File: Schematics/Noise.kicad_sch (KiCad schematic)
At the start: 46 parts, among them J72 Conn_01x04, J73 Conn_01x04, J74 Conn_01x04, Q10 BC547, Q7 BC547, Q8 BC547, Q9 BC547, U116 ADG419BN, U117 TL074

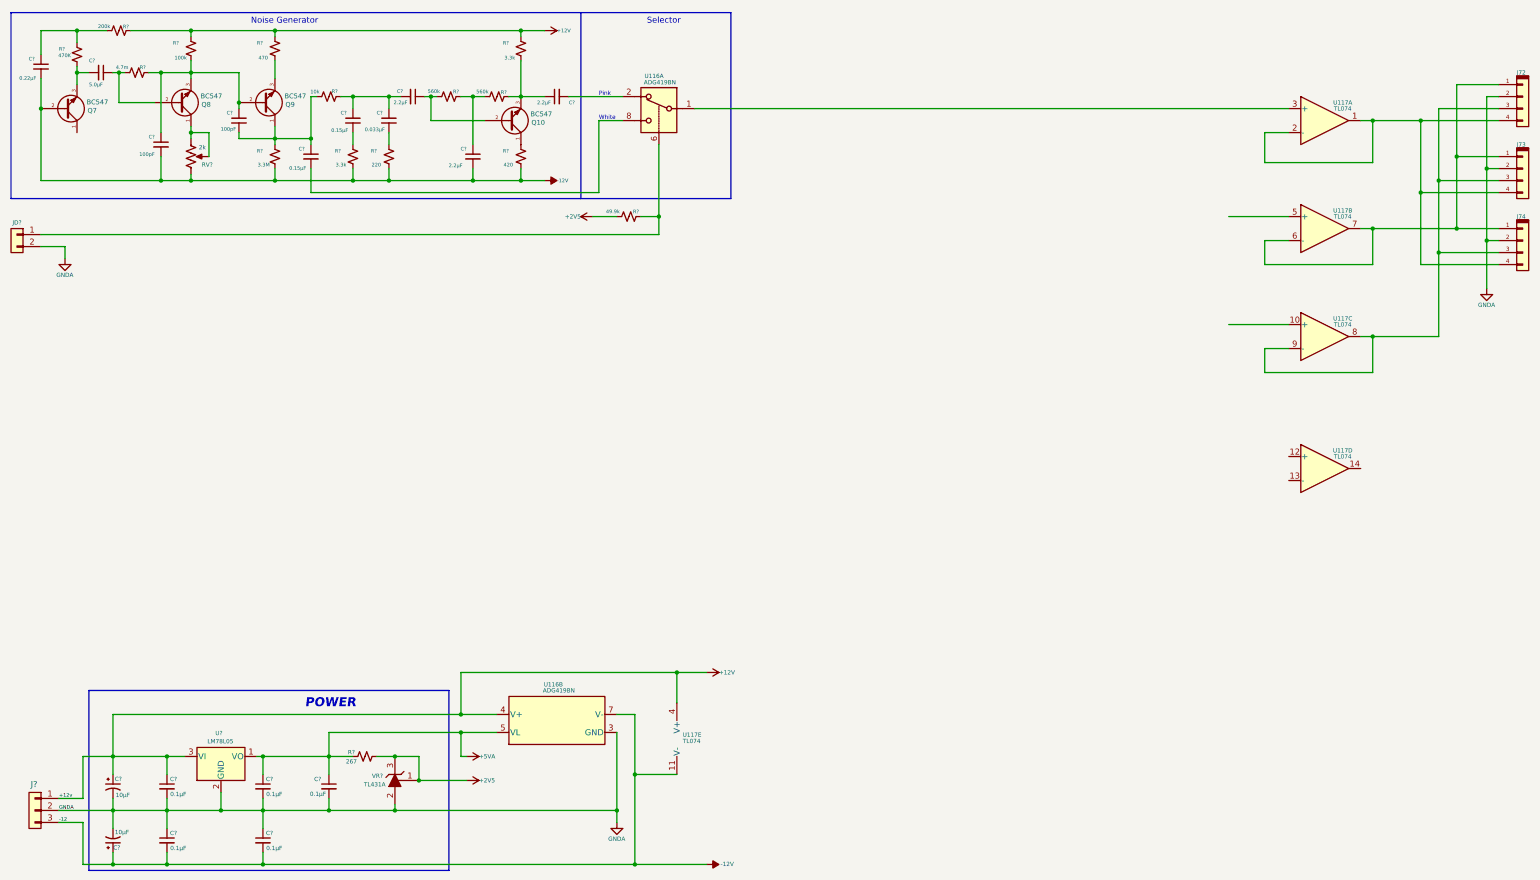
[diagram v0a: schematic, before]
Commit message: sync up first noise board.
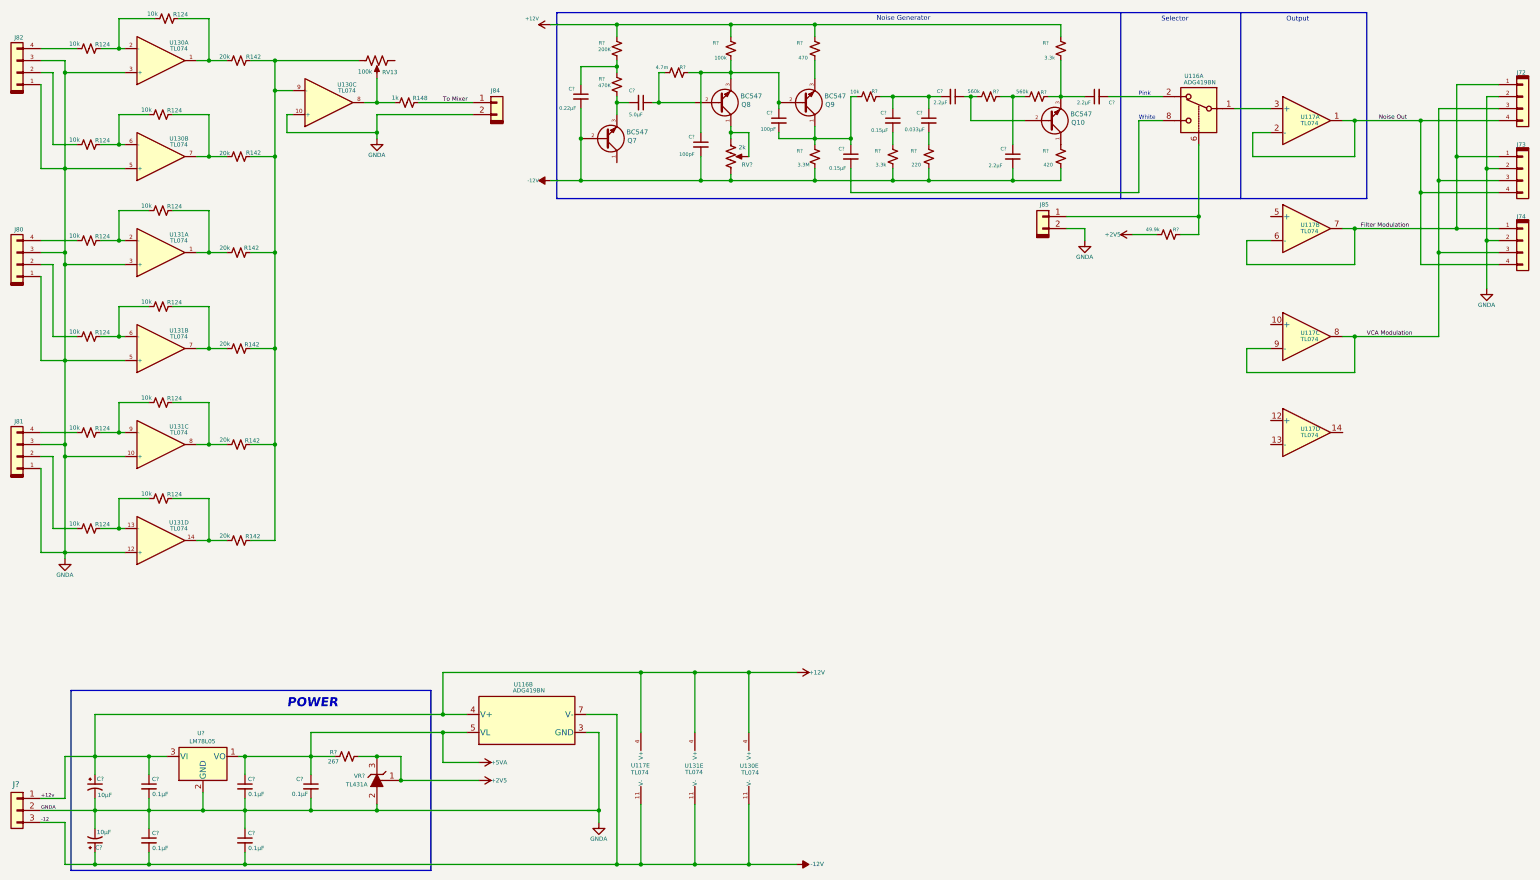
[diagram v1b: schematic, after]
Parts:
- removed JD?: From 12v Analog, symbol Connector_Generic:Conn_01x02
- removed R?: 200k, symbol Device:R_Small_US
- added J80, J81, J82: Conn_01x04, symbol Connector_keyed_kicad_sym:Conn_01x04
- added J84, J85: Conn_01x02, symbol Connector_keyed_kicad_sym:Conn_01x02
- added R124 (x12): 10k, symbol Device:R_Small_US
- added R142 (x6): 20k, symbol Device:R_Small_US
- added R148: 1k, symbol Device:R_Small_US
- added R?: 200K, symbol Device:R_Small_US
- added RV13: 100k, symbol Device:R_Potentiometer_US
- added U130, U131: TL074, symbol Amplifier_Operational:TL074
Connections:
- net +12V: now also R?.1, U130.4 (V+), U131.4 (V+)
- net -12V: now also U130.11 (V-), U131.11 (V-)
- net GNDA: now also J80.1 (Pin_1), J80.3 (Pin_3), J81.1 (Pin_1), J81.3 (Pin_3), J82.1 (Pin_1), J82.3 (Pin_3), J84.2 (Pin_2), J85.2 (Pin_2), U130.10 (+), U130.3 (+), U130.5 (+), U131.10 (+), U131.12 (+), U131.3 (+), U131.5 (+)
- net Filter Modulation: now reaches J72.1 (Pin_1), J73.1 (Pin_1), J74.1 (Pin_1), U117.6 (-), U117.7
- net VCA Modulation: now reaches J72.3 (Pin_3), J73.3 (Pin_3), J74.3 (Pin_3), U117.8, U117.9 (-)
- net Noise Out: now reaches J72.4 (Pin_4), J73.4 (Pin_4), J74.4 (Pin_4), U117.1, U117.2 (-)
- net at R?.1, U116.6: now also J85.1 (Pin_1)
- net at C?.1, R?.1: now also R?.2
- new net: R124.2, R142.1, U131.1
- new net: R124.1, R124.2, U131.2 (-)
- new net: R124.1, R124.2, U131.6 (-)
- new net: R124.2, R142.1, U131.7
- new net: R124.2, R142.1, U131.8
- new net: R142.2, R142.2, R142.2, R142.2, R142.2, R142.2, RV13. (3), U130.9 (-)
- new net: R124.2, R142.1, U131.14
- new net: J80.4 (Pin_4), R124.1
- new net: J82.4 (Pin_4), R124.1
- new net: R124.1, R124.2, U130.2 (-)
- new net: R124.1, R124.2, U131.9 (-)
- new net: R124.2, R142.1, U130.1
- new net: R124.2, R142.1, U130.7
- new net: R124.1, R124.2, U130.6 (-)
- new net: J82.2 (Pin_2), R124.1
- new net: J80.2 (Pin_2), R124.1
- new net: R148.1, RV13. (3), U130.8
- new net: R124.1, R124.2, U131.13 (-)
- new net: J81.4 (Pin_4), R124.1
- new net: J81.2 (Pin_2), R124.1
- new net To Mixer: J84.1 (Pin_1), R148.2
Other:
- note added: "Output"
- title: (none) -> Noise Generator and Mixer
- moved on the sheet: C?, J?, Q10, Q7, Q8, Q9, R?, RV?, U116A, U116B, U117A, U117B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
